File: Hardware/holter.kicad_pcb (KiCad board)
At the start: 6 copper layers, 33.5 x 48 mm, 262 parts, among them CN1 2TAP, CN2 2TAP, CN3 3TAP, IC1 256kx8, M1 USB_Power_Module, M2 USB_Power_Module, P1 CONN_01X07, P2 PROG, P3 SCREW, P4 BAT-, Q1 PMF170XP, Q2 PMF170XP, Q3 NTR4101PT1G, Q4 PMF170XP, Q5 PMF170XP, U1 TXB0106, U10 TS5A3159, U11 TS5A3159, U12 ESD_PROTECTOR, U13 ESD_PROTECTOR, U14 ESD_PROTECTOR, U15 ESD_PROTECTOR, U16 ESD_PROTECTOR, U17 ESD_PROTECTOR, U18 ESD_PROTECTOR, U19 ESD_PROTECTOR, U2 TXB0106, U20 ESD_PROTECTOR, U21 ESD_PROTECTOR, U22 ESD_PROTECTOR, U23 ESD_PROTECTOR, U24 TLV61220, U25 TLV61220, U26 TLV61220, U27 LM3671, U28 DS2710, U29 LIS2DH12, U3 TiWi-uB2, U4 STM32F4x1_64, U5 uSD, U6 ADS1298, U7 USBULC6-2M6, U8 USB2641, U9 OPA379, X1 32768, Y1 24 MHz, Y2 10 MHz

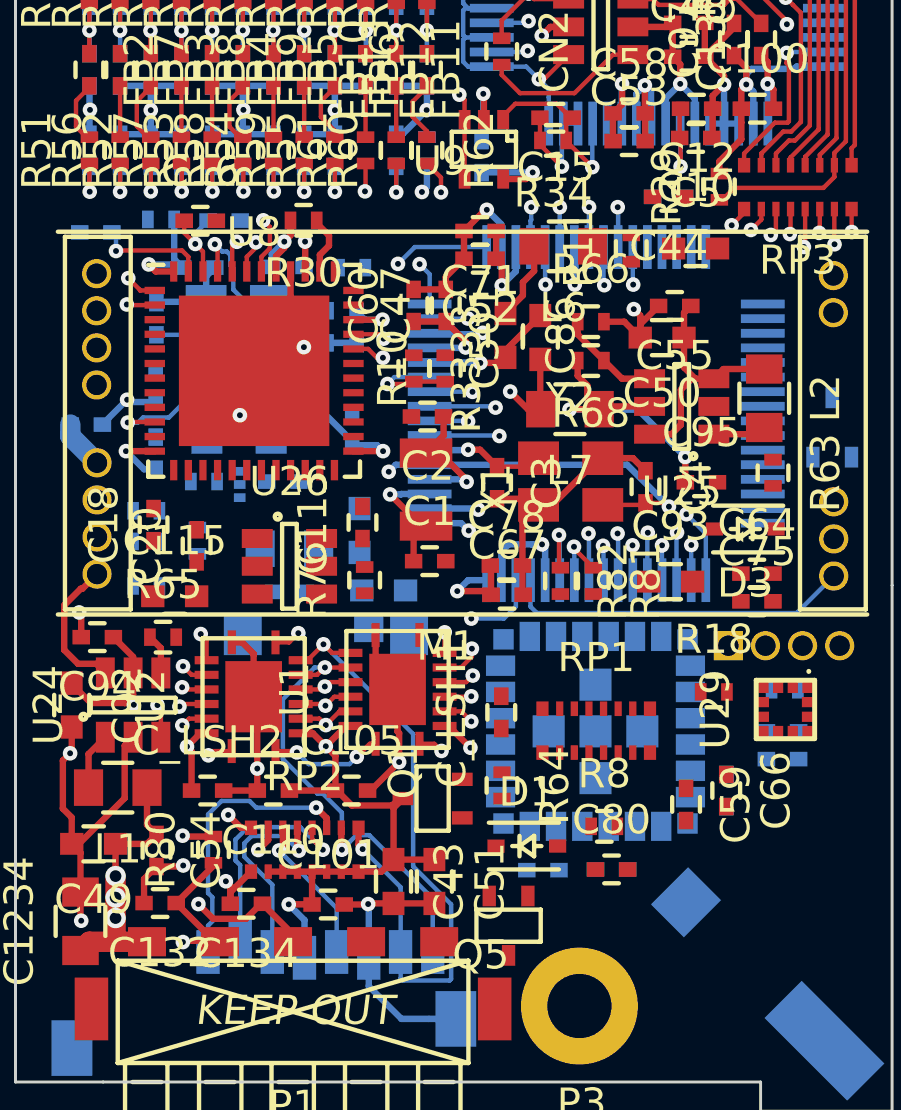
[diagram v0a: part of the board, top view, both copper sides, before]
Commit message: Routing attempt.
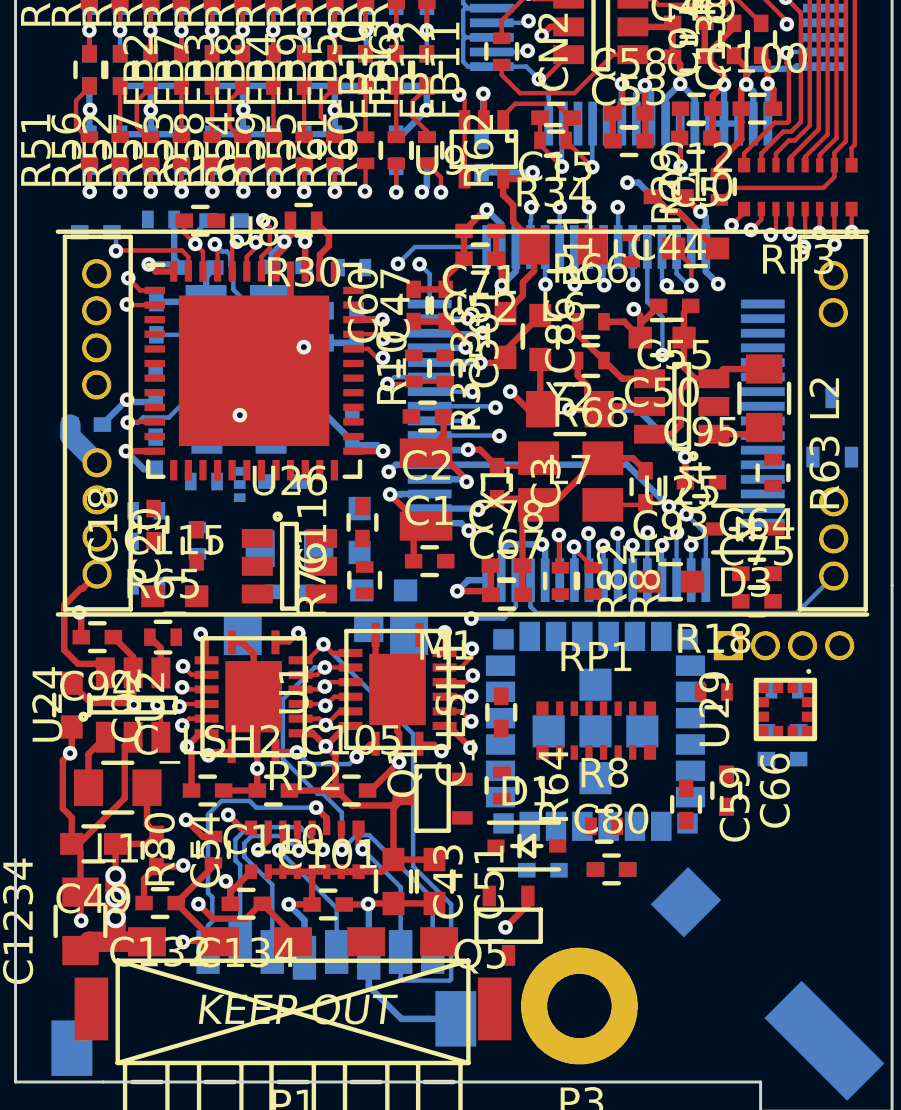
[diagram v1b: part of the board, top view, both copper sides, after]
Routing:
- net VCPU: track 10.3 -> 34.8 mm, vias 3 -> 5
- net +2.8VA: track 30.3 -> 48.5 mm
- net ~ECG_PWDN: track 4.24 -> 22.2 mm
- net +3V3: track 19.4 -> 37.1 mm, vias 6 -> 7
- net +1V8: track 15.5 -> 28.4 mm
- net ~ECG_RST: track 2.57 -> 13.2 mm
- net DIFF_SEL: track 3.01 -> 13.5 mm
- net ECG_START: track 2.61 -> 12.0 mm
- net ~ECG_DRDY: track 2.11 -> 9.63 mm
- net GND: track 173.1 -> 179.6 mm, vias 40 -> 41
- net SD_CPU: track 0.96 -> 4.87 mm, vias 1 -> 2
- net Net-(C5-Pad1): track 0.00 -> 3.11 mm, vias 0 -> 1
- net ~CARD_DET: track 0.00 -> 1.38 mm, vias 0 -> 1
